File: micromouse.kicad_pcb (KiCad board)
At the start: 2 copper layers, 115 x 122.4 mm, 16 parts, among them J1 XT60-M, SW1 SW_SPST, SW2 SW_Push, SW3 SW_SPDT_312, SW4 SW_Push, U1 BUCK, U2 STM32 Blackpill, U3 N20 encoder right, U4 N20 encoder left, U5 TB6612FNG, U6 VL53L0X left, U7 VL53L0X right, U8 VL53L0X middle, U9 oled i2c

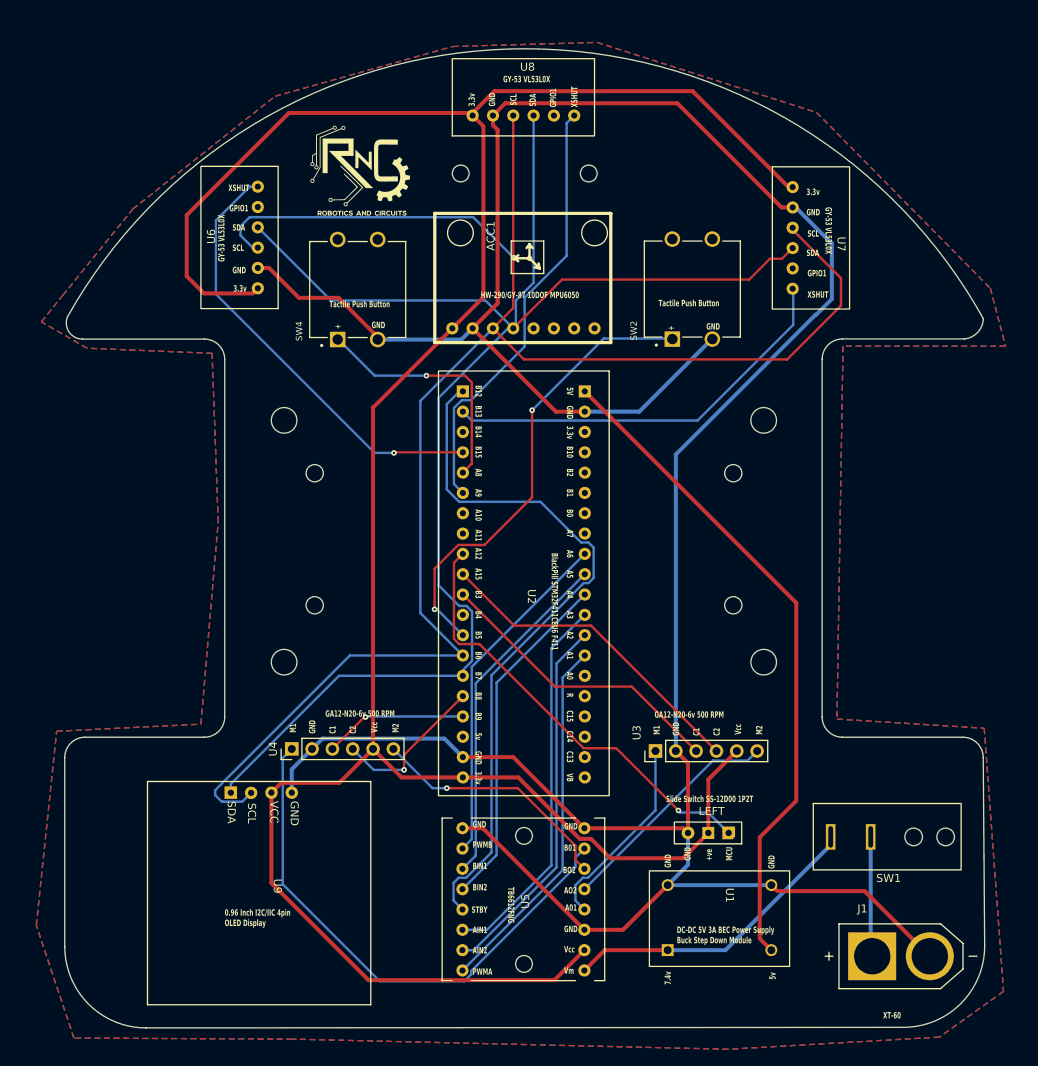
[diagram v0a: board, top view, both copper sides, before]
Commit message: final
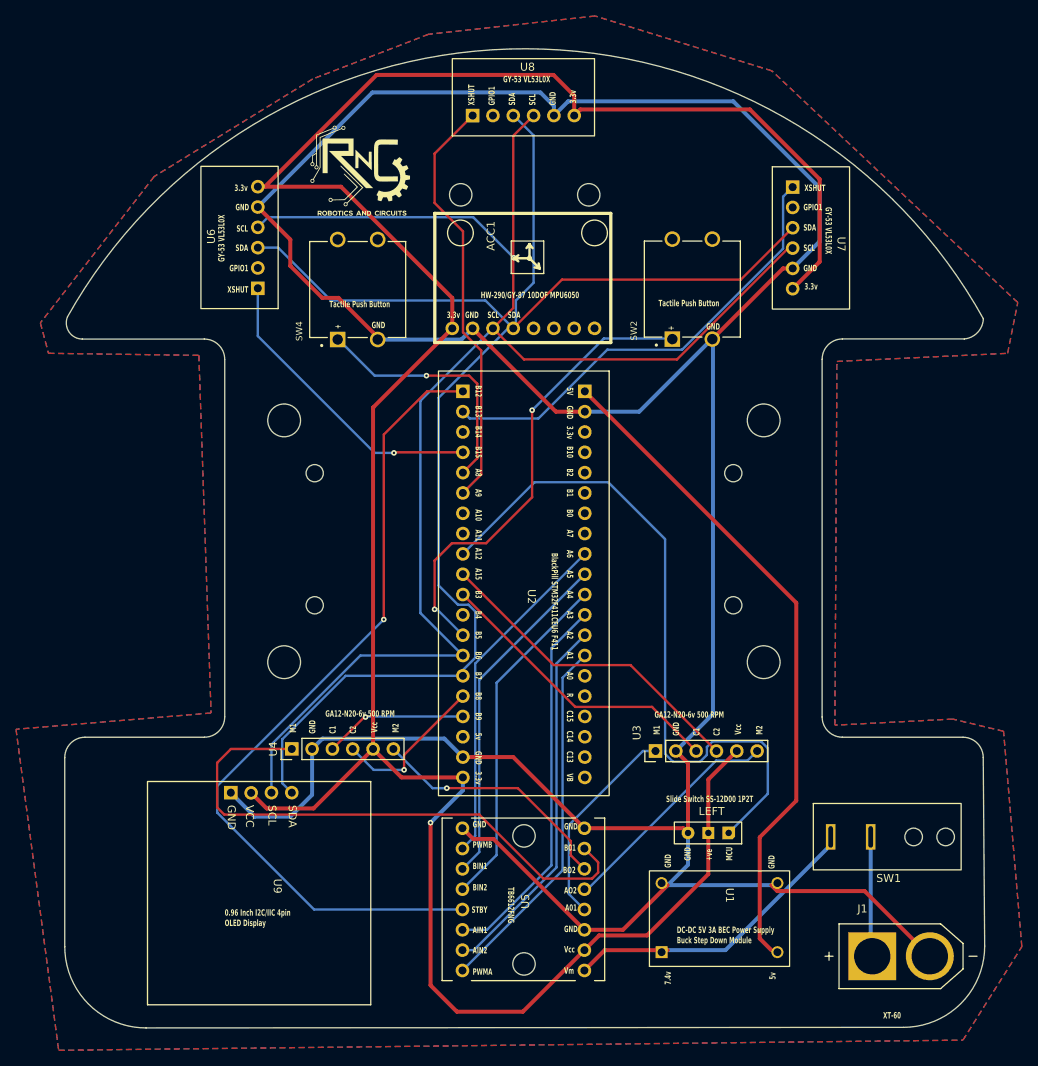
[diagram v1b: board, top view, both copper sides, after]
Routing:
- net slide_SW: track 55.5 -> 86.6 mm, vias 1 -> 0
- net SCL: track 219.2 -> 189.6 mm
- net GND: track 366.2 -> 395.0 mm
- net XSHUT 3: track 55.3 -> 37.7 mm
- net STBY: track 88.6 -> 103.7 mm, vias 0 -> 1
- net 3.3v: track 323.3 -> 308.8 mm, vias 0 -> 1
- net XSHUT 1: track 51.3 -> 57.9 mm
- net BO1: track 67.9 -> 71.0 mm
- net XSHUT 2: track 54.5 -> 53.3 mm
- net AO1: track 24.8 -> 26.0 mm
- net push button: track 30.6 -> 31.5 mm
- net SDA: track 190.0 -> 189.3 mm
- net push button 1: track 57.9 -> 58.5 mm
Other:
- outline, holes or cut-outs redrawn
